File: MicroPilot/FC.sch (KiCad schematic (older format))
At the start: 29 parts

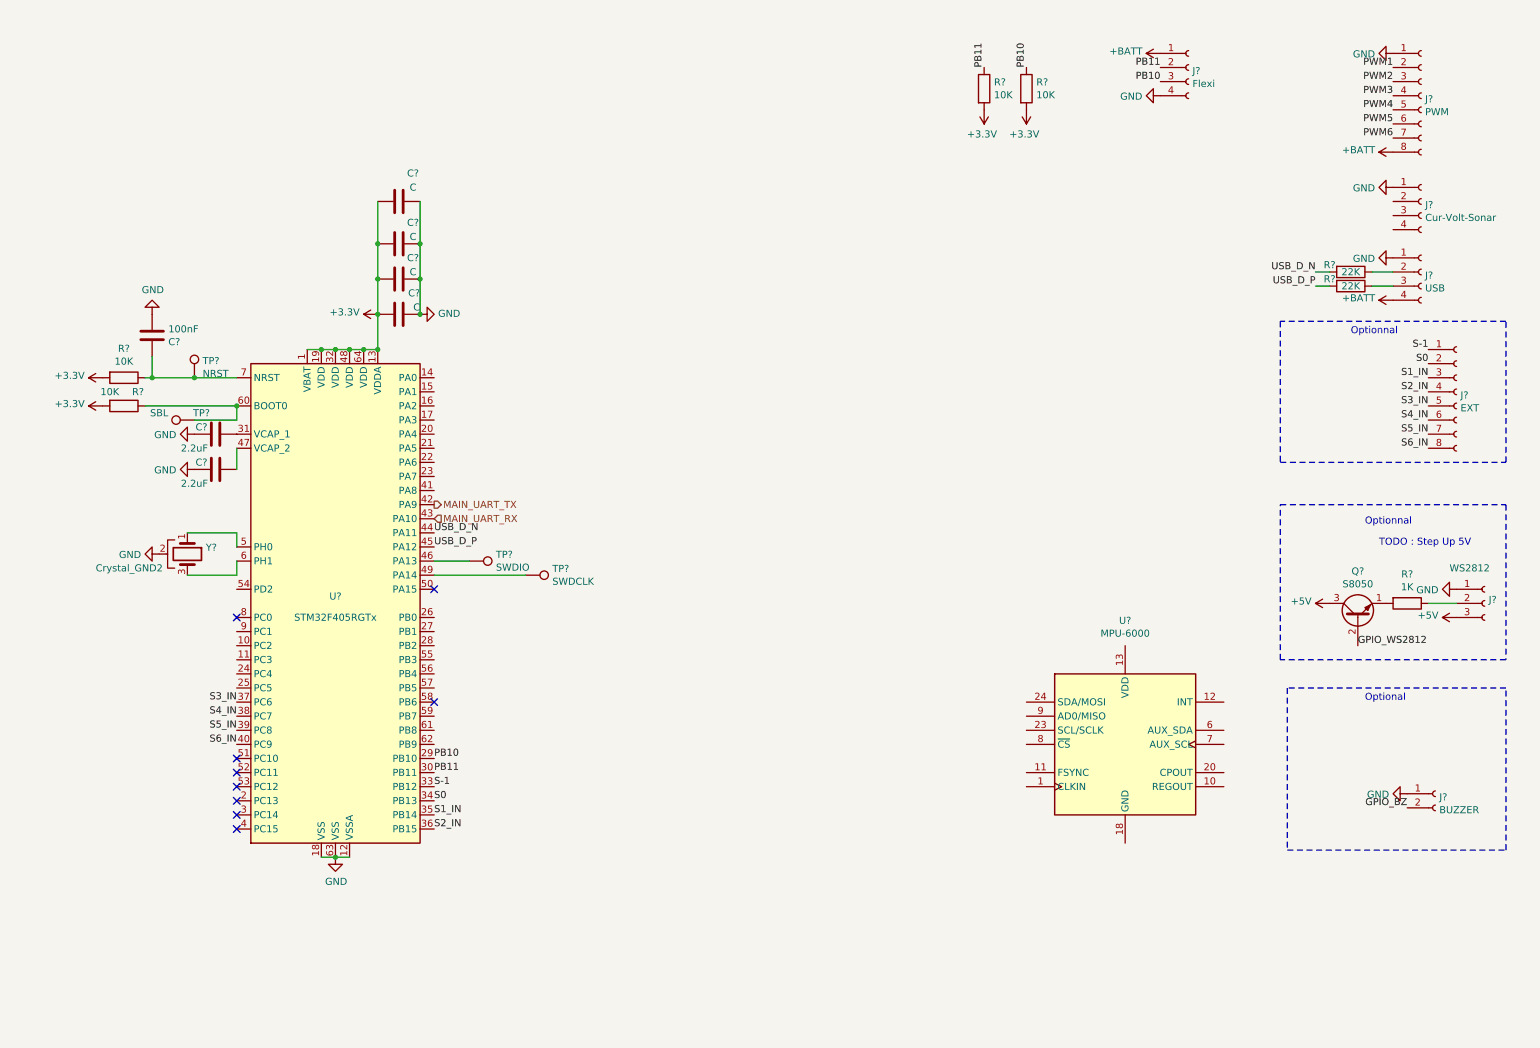
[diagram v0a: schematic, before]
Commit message: MicroPilot schematic done
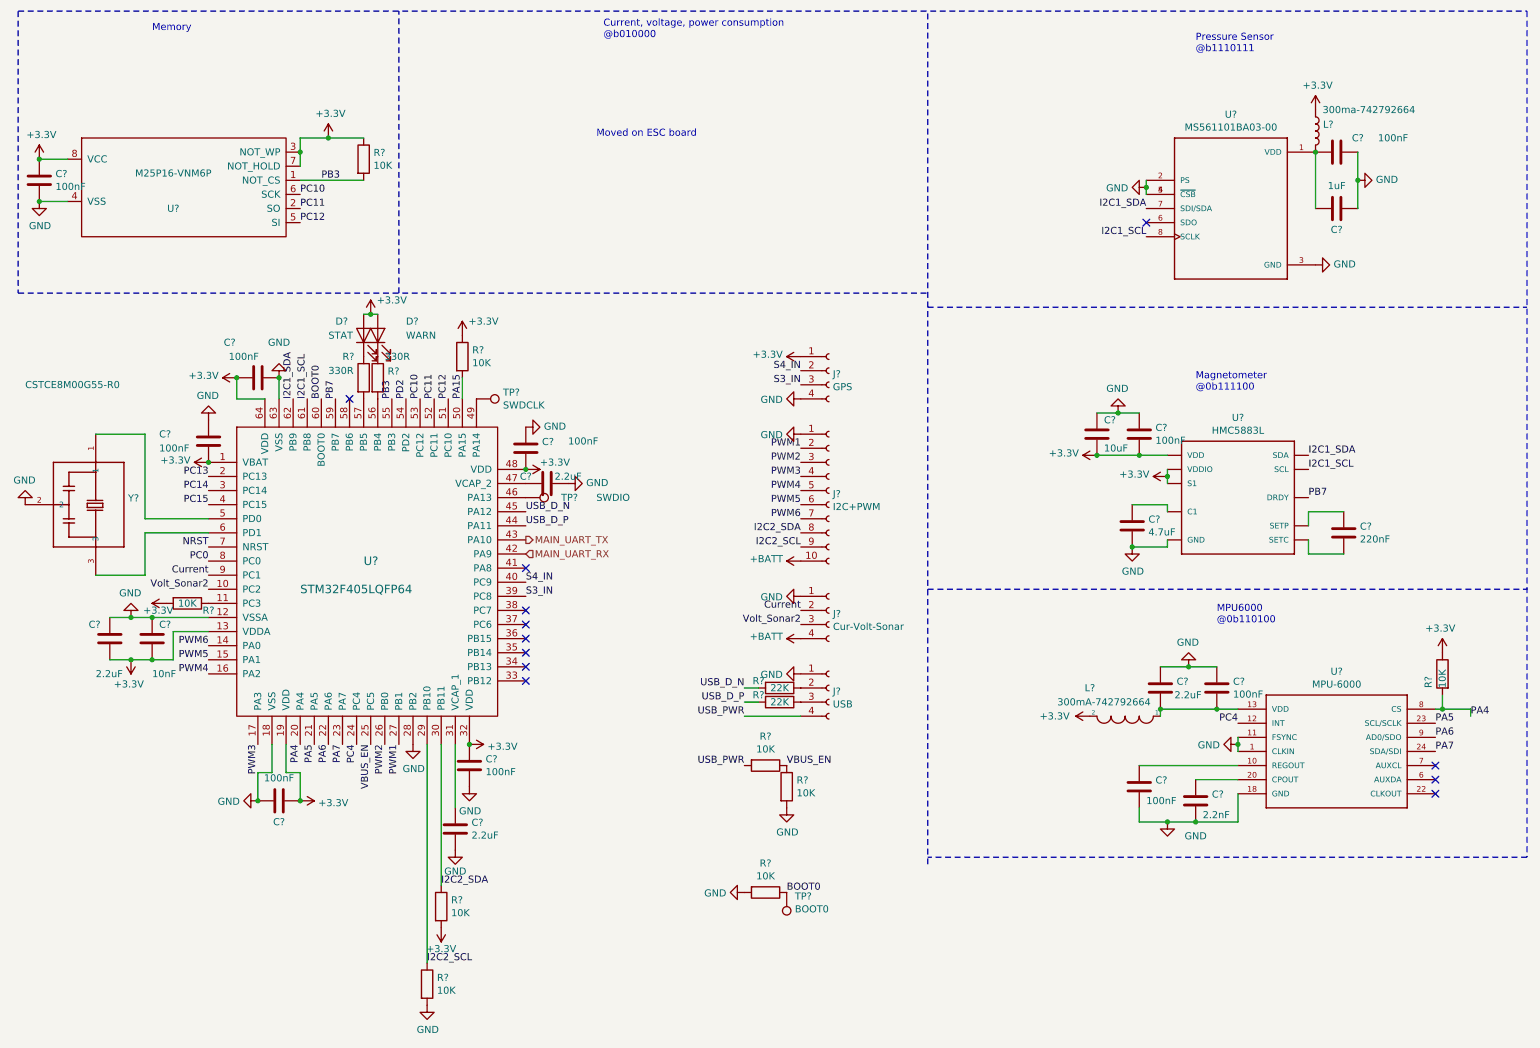
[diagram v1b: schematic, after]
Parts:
- removed C? (x4): C, symbol Device:C
- removed C?: 100nF, symbol Device:C
- removed C? (x2): 2.2uF, symbol Device:C
- removed J?: PWM, symbol Connector:Conn_01x08_Female
- removed J?: EXT, symbol Connector:Conn_01x08_Female
- removed J?: WS2812, symbol Connector:Conn_01x03_Female
- removed J?: BUZZER, symbol Connector:Conn_01x02_Female
- removed J?: Flexi, symbol Connector:Conn_01x04_Female
- removed Q?: S8050, Package_TO_SOT_THT:TO-92_Inline, symbol Transistor_BJT:S8050
- removed R?: 1K, symbol Device:R
- removed R? (x4): 10K, symbol Device:R
- removed TP?: NRST, symbol Connector:TestPoint
- removed TP?: SBL, symbol Connector:TestPoint
- removed U?: MPU-6000, Sensor_Motion:InvenSense_QFN-24_4x4mm_P0.5mm, symbol Sensor_Motion:MPU-6000
- removed U?: STM32F405RGTx, Package_QFP:LQFP-64_10x10mm_P0.5mm, symbol MCU_ST_STM32F4:STM32F405RGTx
- removed Y?: Crystal_GND2, symbol Device:Crystal_GND2
- added C?: 2.2nF, symbol Device:C
- added C? (x10): 100nF, symbol Device:C
- added C? (x4): 2.2uF, symbol Device:C
- added C?: 220nF, symbol Device:C
- added C?: 4.7uF, symbol Device:C
- added C?: 10uF, symbol Device:C
- added C?: 10nF, symbol Device:C
- added C?: 1uF, symbol Device:C
- added D?: WARN, symbol Device:LED
- added D?: STAT, symbol Device:LED
- added J?: GPS, symbol Connector:Conn_01x04_Female
- added J?: I2C+PWM, symbol Connector:Conn_01x10_Female
- added L?: 300mA-742792664, symbol pspice:INDUCTOR
- added L?: 300ma-742792664, symbol Device:L
- added R? (x9): 10K, symbol Device:R
- added R? (x2): 330R, symbol Device:R
- added TP?: BOOT0, symbol Connector:TestPoint
- added U?: M25P16-VNM6P, symbol M25P16:M25P16-VNM6P
- added U?: HMC5883L, LPCC-16, symbol HMC5883L:HMC5883L
- added U?: MS561101BA03-00, SON125P500X300X100-8N, symbol MS561101BA03-00:MS561101BA03-00
- added U?: MPU-6000, QFN-24-TESTING, symbol MPU-6000:MPU-6000
- added U?: STM32F405LQFP64, symbol stm32f405lqfp64:STM32F405LQFP64
- added Y?: CSTCE8M00G55-R0, OSC_CSTCE8M00G55-R0, symbol CSTCE8M00G55-R0:CSTCE8M00G55-R0
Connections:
- net +3V3: now also C?.1, C?.1, C?.1, C?.2, C?.2, C?.2, C?.2, C?.2, C?.2, C?.2, D?.2 (A), D?.2 (A), J?.1 (Pin_1), L?.1, L?.2, R?.1, R?.1, R?.1, R?.2, R?.2, U?.1 (VBAT), U?.13 (VDDA), U?.13 (VDDIO), U?.19 (VDD), U?.2 (VDD), U?.3 (NOT_WP), U?.32 (VDD), U?.4 (S1), U?.48 (VDD), U?.64 (VDD), U?.7 (NOT_HOLD), U?.8 (VCC)
- net +BATT: now also J?.4 (Pin_4), J?.10 (Pin_10); no longer J?.4 (Pin_4)
- net GND: now also C?.1, C?.1, C?.1, C?.1, C?.1, C?.1, C?.1, C?.1, C?.1, C?.1, C?.1, C?.1, C?.2, C?.2, C?.2, C?.2, C?.2, C?.2, C?.2, J?.1 (Pin_1), J?.4 (Pin_4), R?.2, R?.2, R?.2, U?.1 (CLKIN), U?.11 (FSYNC), U?.11 (GND), U?.12 (VSSA), U?.18 (GND), U?.18 (VSS), U?.2 (PS), U?.28 (PB2), U?.3 (GND), U?.4 (VSS), U?.4 (~CSB~), U?.5 (~CSB~), U?.63 (VSS), U?.9 (GND), Y?.2
- net MAIN_UART_RX: now also U?.42 (PA9)
- net MAIN_UART_TX: now also U?.43 (PA10)
- net PWM1: now also J?.2 (Pin_2), U?.27 (PB1)
- net PWM2: now also J?.3 (Pin_3), U?.26 (PB0)
- net PWM3: now also J?.4 (Pin_4), U?.17 (PA3)
- net PWM4: now also J?.5 (Pin_5), U?.16 (PA2)
- net PWM5: now also J?.6 (Pin_6), U?.15 (PA1)
- net PWM6: now also J?.7 (Pin_7), U?.14 (PA0)
- net S3_IN: now also J?.3 (Pin_3), U?.39 (PC8)
- net S4_IN: now also J?.2 (Pin_2), U?.40 (PC9)
- net USB_D_N: now also U?.45 (PA12)
- net USB_D_P: now also U?.44 (PA11)
- net Current: now reaches J?.2 (Pin_2)
- net Current: now also U?.9 (PC1)
- net Volt_Sonar2: now reaches J?.3 (Pin_3)
- net Volt_Sonar2: now also U?.10 (PC2)
- net at TP?.1: now also U?.49 (PA14)
- net at TP?.1: now also U?.46 (PA13)
- new net: C?.1, U?.10 (C1)
- new net: C?.2, U?.12 (SETC)
- new net: C?.1, U?.8 (SETP)
- new net: C?.2, C?.2, L?.2, U?.1 (VDD)
- new net: C?.1, U?.10 (REGOUT)
- new net: C?.2, C?.2, L?.1, U?.13 (VDD)
- new net: C?.1, U?.20 (CPOUT)
- new net: R?.1, U?.11 (PC3)
- new net: C?.1, U?.31 (VCAP_1)
- new net: C?.2, U?.47 (VCAP_2)
- new net: U?.5 (PD0), Y?.1
- new net: R?.2, U?.56 (PB4)
- new net: R?.2, U?.57 (PB5)
- new net: U?.6 (PD1), Y?.3
- new net: D?.1 (K), R?.1 (x2)
- new net BOOT0: R?.1, TP?.1, U?.60 (BOOT0)
- new net I2C1_SCL: U?.1 (SCL), U?.61 (PB8), U?.8 (SCLK)
- new net I2C1_SDA: U?.16 (SDA), U?.62 (PB9), U?.7 (SDI/SDA)
- new net I2C2_SCL: J?.9 (Pin_9), R?.1, U?.29 (PB10)
- new net I2C2_SDA: J?.8 (Pin_8), R?.1, U?.30 (PB11)
- new net NRST: U?.7 (NRST)
- new net PA15: R?.2, U?.50 (PA15)
- new net PA4: R?.2, U?.20 (PA4), U?.8 (CS)
- new net PA5: U?.21 (PA5), U?.23 (SCL/SCLK)
- new net PA6: U?.22 (PA6), U?.9 (AD0/SDO)
- new net PA7: U?.23 (PA7), U?.24 (SDA/SDI)
- new net PB3: R?.2, U?.1 (NOT_CS), U?.55 (PB3)
- new net PB7: U?.15 (DRDY), U?.59 (PB7)
- new net PC0: U?.8 (PC0)
- new net PC10: U?.53 (PC12), U?.6 (SCK)
- new net PC11: U?.2 (SO), U?.52 (PC11)
- new net PC12: U?.5 (SI), U?.51 (PC10)
- new net PC13: U?.2 (PC13)
- new net PC14: U?.3 (PC14)
- new net PC15: U?.4 (PC15)
- new net PC4: U?.12 (INT), U?.24 (PC4)
- new net PD2: U?.54 (PD2)
- new net USB_PWR: J?.4 (Pin_4), R?.2
- new net VBUS_EN: R?.1, R?.1, U?.25 (PC5)
- no-connect marks 9 -> 12
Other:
- note added: "Current, voltage, power consumption\n@b010000"
- note added: "MPU6000\n@0b110100"
- note added: "Magnetometer\n@0b111100"
- note added: "Memory"
- note added: "Moved on ESC board"
- note added: "Pressure Sensor\n@b1110111"
- note removed: "Optional"
- note removed: "Optionnal"
- note removed: "TODO : Step Up 5V"
- moved on the sheet: J?, R?, TP?
